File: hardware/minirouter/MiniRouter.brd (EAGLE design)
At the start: 96.5 x 55.9 mm, 50 parts, among them J0 CON-MATENLOK, J1 AVR_PROG, J2 RJ45-8PTH, J3 RJ45-8PTH, J4 RJ45-8PTH, J5 RASPBERRY-PI_REV2, Q1 NMOS, Q2 NMOS, Q3 NMOS, U1 ATMEGA168, U2 AOZ1242SMD, U3 DS1307SO8, Y1 32.768kHz

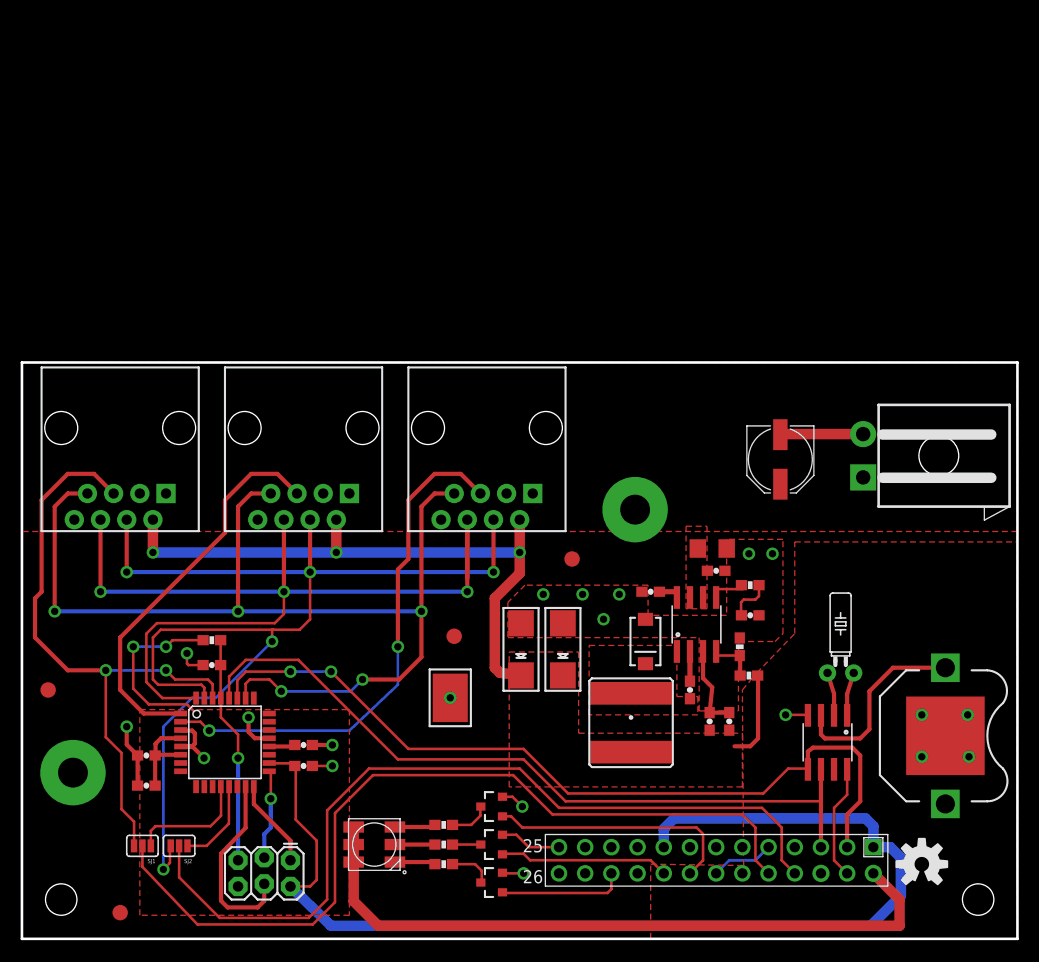
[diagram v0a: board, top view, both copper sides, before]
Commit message: Checking in the latest schematics for the kickstarter
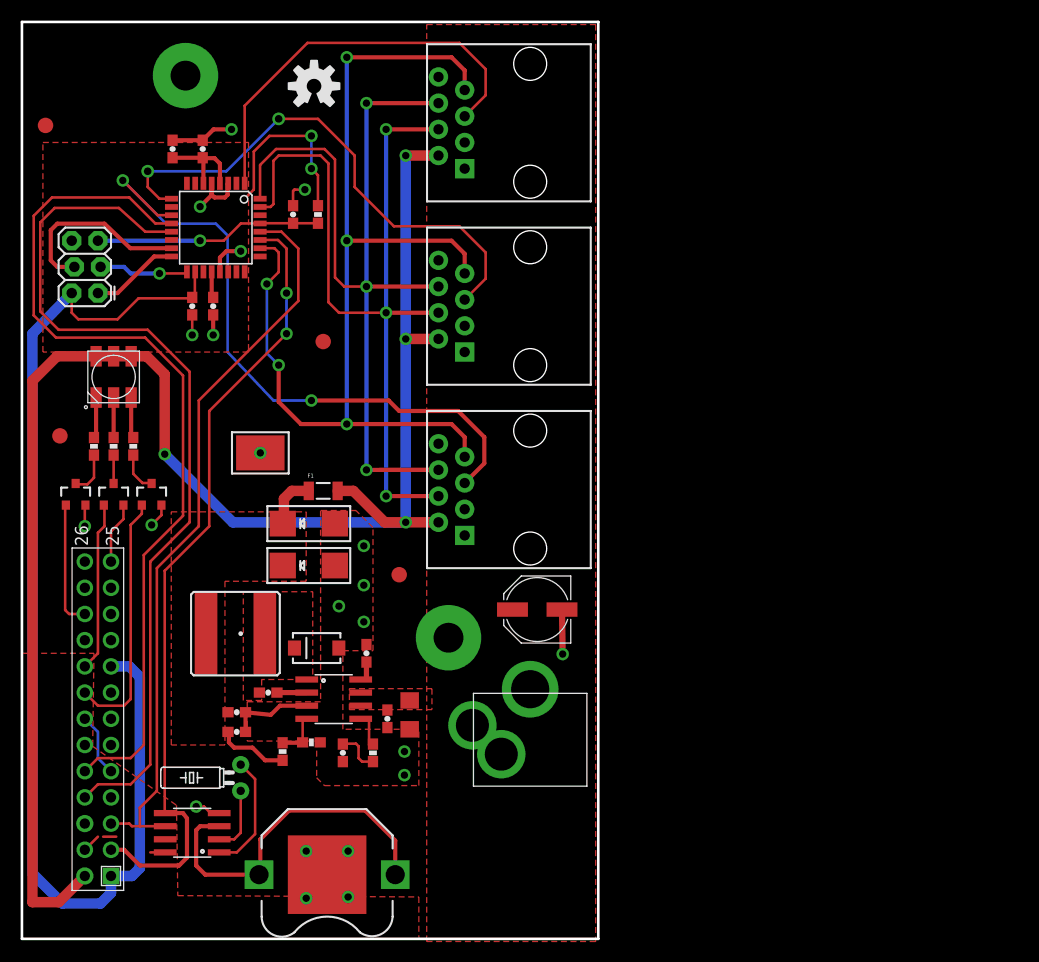
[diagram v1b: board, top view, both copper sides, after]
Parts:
- removed CR1220: 3V, SparkFun-Electromechanical:BATTCON_12MM_PTH
- removed J0: CON-MATENLOK, pierre:MINIMATENLOK-2RA
- removed JP6, JP7: STAND-OFFTIGHT, SparkFun-Electromechanical:STAND-OFF-TIGHT
- removed SJ1, SJ2: (no value), SparkFun-Passives:SJ_3_PASTE1&2
- added F1: PTCSMD, SparkFun:PTC-1206
- added J6: 2.1MMJACKTHM, pierre:PJ-102A
- added J7: 3V, SparkFun-Electromechanical:BATTCON_12MM_PTH
- moved U$46 95.7 mm to (28.3, 82.7)
- moved JP4 76.7 mm to (2.29, 78.9), turned to 90 degrees
- moved U3 62.2 mm to (16.5, 10.3), turned to 90 degrees
- moved C3 61.8 mm to (14.6, 76.6), turned to 90 degrees
- moved C5 59.1 mm to (17.5, 76.6), turned to 90 degrees
- moved Y1 59.0 mm to (21.2, 15.6), turned to 90 degrees
- moved J1 58.1 mm to (7.37, 62.6), turned to 90 degrees
- moved Q1 55.2 mm to (5.21, 43.1), turned to 0 degrees
- moved R1 52.8 mm to (6.99, 47.8), turned to 270 degrees
- moved D2 51.9 mm to (8.89, 54.5), turned to 270 degrees
- moved R2 50.1 mm to (8.89, 47.8), turned to 270 degrees
- moved Q2 50.0 mm to (8.89, 43.1), turned to 0 degrees
- moved U1 49.9 mm to (18.8, 69.0), turned to 270 degrees
- moved J2 49.6 mm to (49.3, 79.1), turned to 90 degrees
- moved C15 47.8 mm to (20.8, 20.1), turned to 0 degrees
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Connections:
- removed net RX0: J2.5, SJ1.3, U1.30
- removed net U_RX: SJ1.1, U1.12
- removed net U_TX: SJ2.1, U1.13
- new net N$5: C14.1, C15.1, C16.+, C4.+, F1.1, L1.P$2, R4.2
- new net RX3: J4.5, U1.11
- net 5V: now also F1.2; no longer C14.1, C15.1, C16.+, C4.+, L1.P$2, R4.2
- net BAT1+: now also J7.VCC@1; no longer CR1220.VCC@1
- net GND: now also J6.RING, J6.RING_SW, J7.GND; no longer CR1220.GND, J0.2
- net RPI_RX: now also U1.12; no longer SJ1.2
- net RPI_TX: now also U1.13; no longer SJ2.2
- net RX1: now also J2.5; no longer J3.5
- net RX2: now also J3.5, U1.9; no longer J4.5, U1.2
- net TX: no longer SJ2.3
- net VIN: now also J6.TIP; no longer J0.1
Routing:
- net RX3: track 0.00 -> 63.4 mm, vias 0 -> 2
- net RX0: track 61.0 -> 0.00 mm, vias 2 -> 0
- net TX: track 113.3 -> 81.7 mm, vias 5 -> 3
- net BAT1+: track 19.1 -> 34.5 mm
- net 5V: track 150.5 -> 165.9 mm, vias 3 -> 4
- net N$5: track 0.00 -> 12.2 mm
- net U_RX: track 11.7 -> 0.00 mm
- net U_TX: track 8.50 -> 0.00 mm
- net N$6: track 4.21 -> 11.5 mm
- net RPI_TX: track 81.5 -> 87.1 mm
- net RPI_RX: track 82.0 -> 85.9 mm
- net GND: track 61.1 -> 57.8 mm, vias 20 -> 21
- net RPI_SDA: track 80.0 -> 77.0 mm
- net N$1: track 4.21 -> 6.41 mm
- net RX1: track 38.3 -> 39.9 mm
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- added copper zone on layer 1, net N$5
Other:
- board size 96.5 x 55.9 mm -> 55.9 x 88.9 mm
- board text added: "1"
- board text added: "2"
- board text added: "24VDC"
- board text added: "3"
- board text added: "3A"
- board text added: "F1"
- board text added: "miniRouter v2"
- board text removed: "24VDC 3A In"
- board text removed: "J0"
- board text removed: "MiniRouter v1"
- board text removed: "Pump 1"
- board text removed: "Pump 2"
- board text removed: "Pump 3"
